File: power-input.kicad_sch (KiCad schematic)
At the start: 27 parts, among them J1 PJ-018, J2 MDT420E03002, Q1 TSM9409CS, Q2 TSM9409CS, Q3 TSM9409CS, U1 TPS54331DRG4

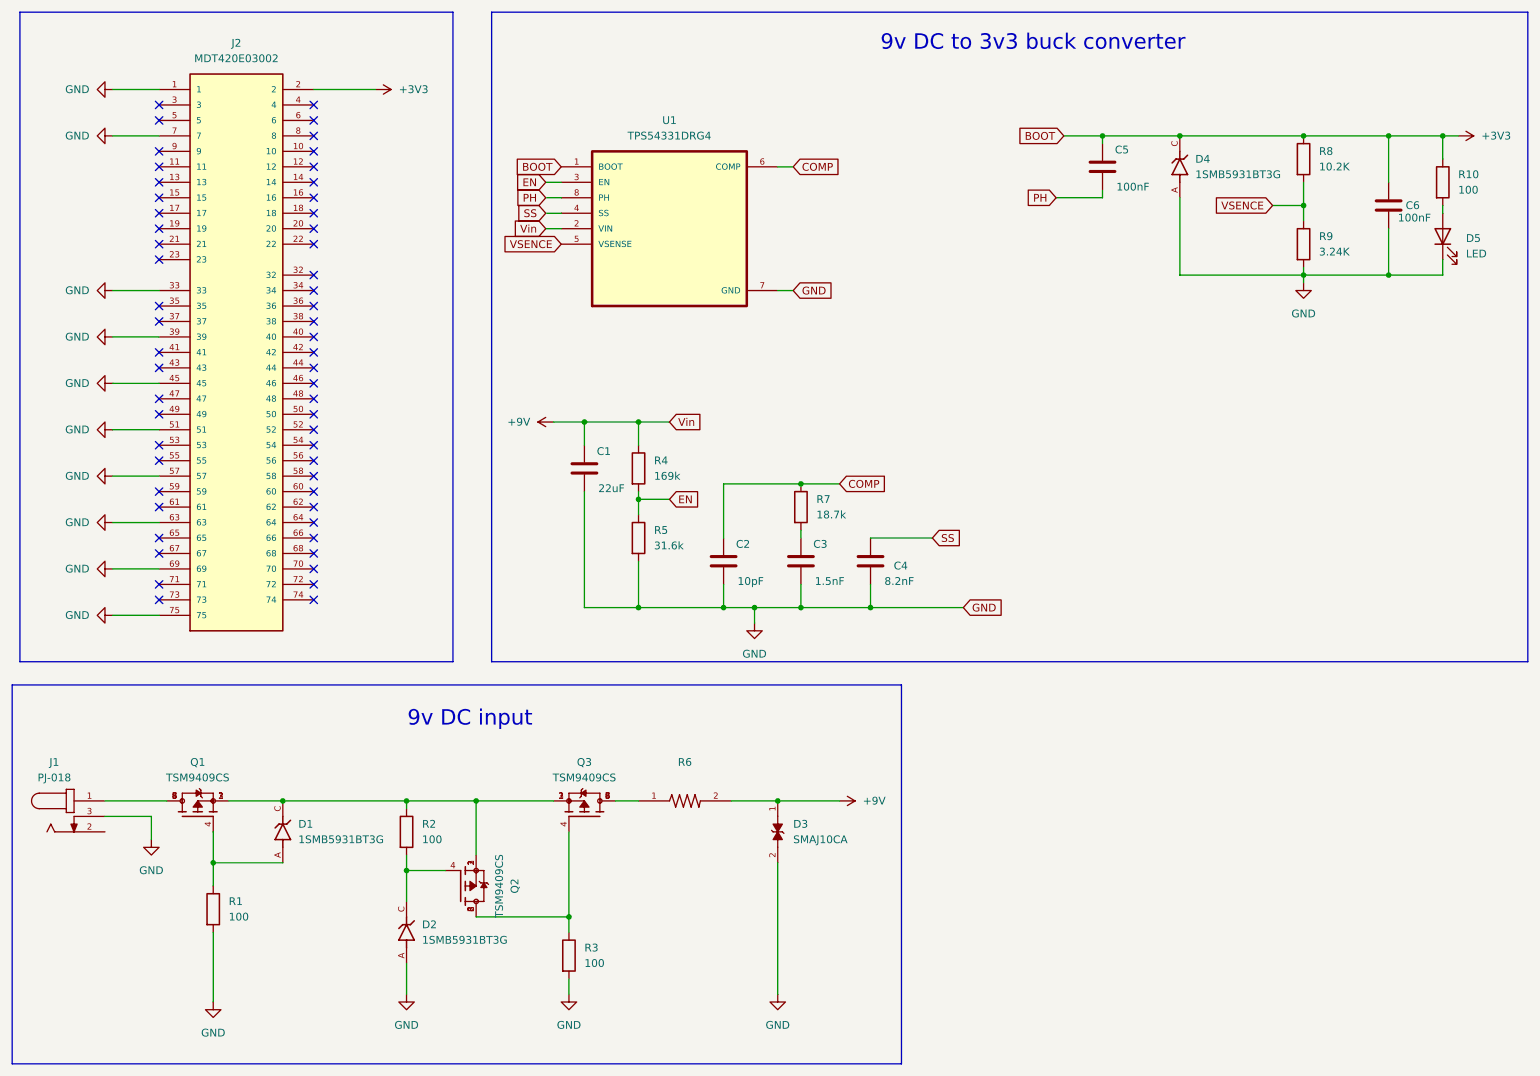
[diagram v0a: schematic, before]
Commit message: Add BMS
Signed-off-by: JeffMboya <jangina.mboya@gmail.com>
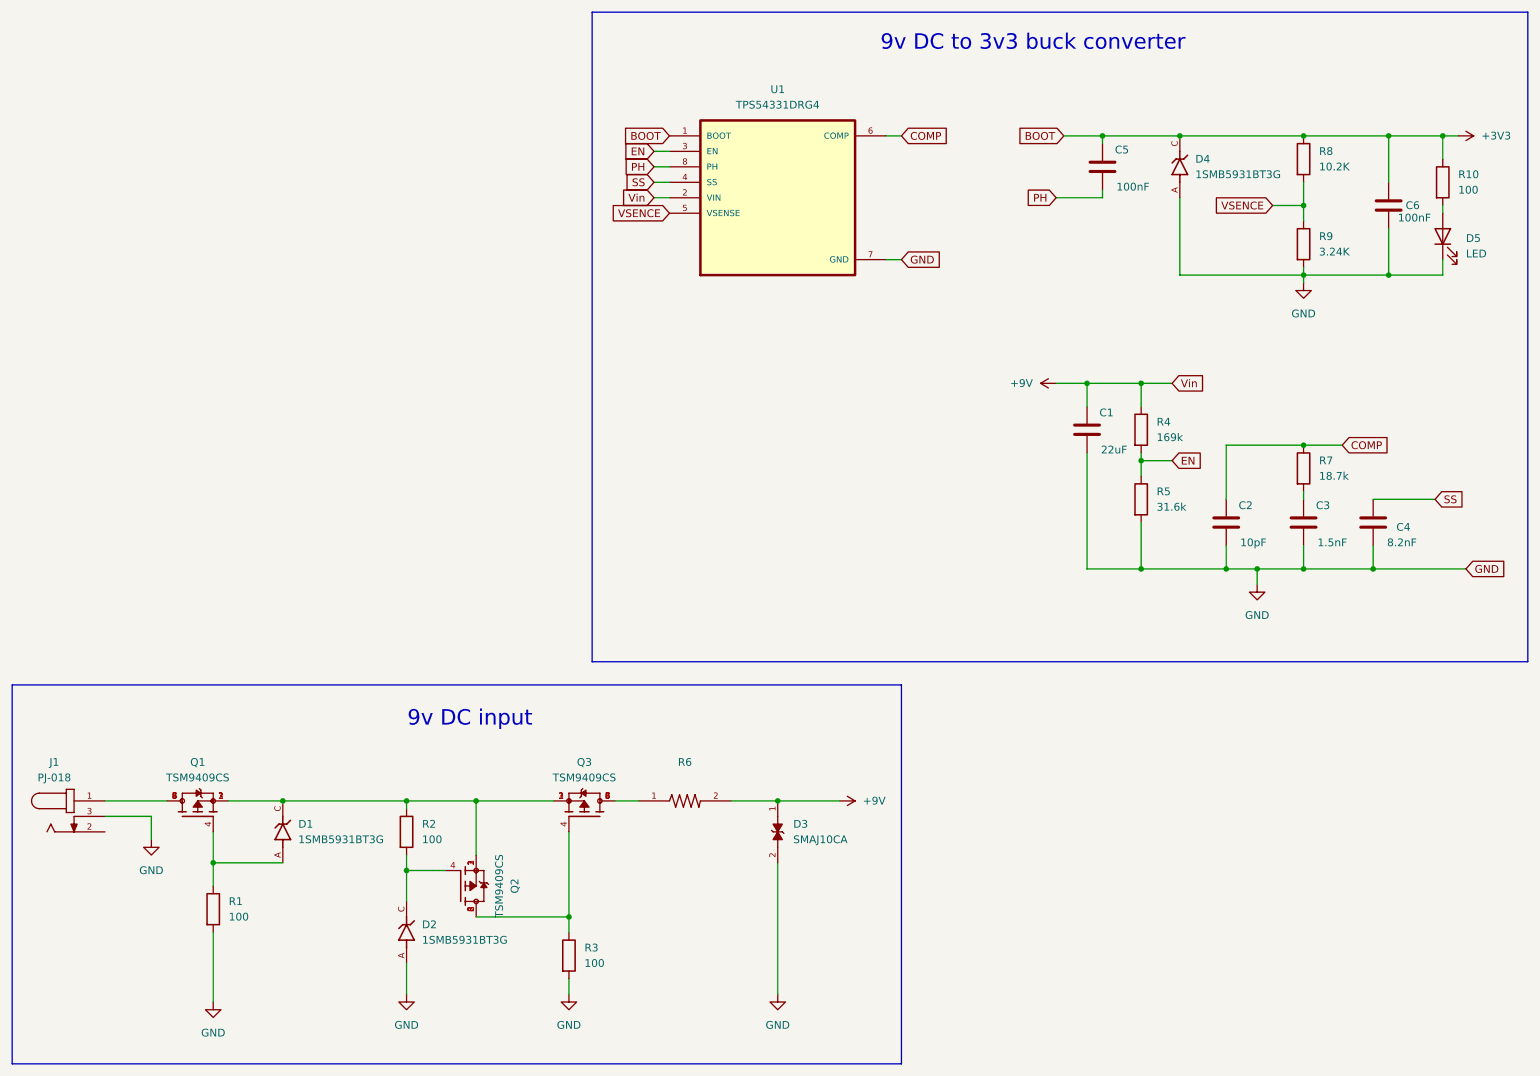
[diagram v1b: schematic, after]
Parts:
- removed J2: MDT420E03002, MDT420E03002:AMPHENOL_MDT420E03002, symbol MDT420E03002:MDT420E03002
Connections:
- no-connect marks 56 -> 0
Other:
- company: (none) -> ABTTRACT MACHINES
- title: (none) -> M.2 E-KEY SOCKET
- moved on the sheet: C1, C2, C3, C4, R4, R5, R7, U1
